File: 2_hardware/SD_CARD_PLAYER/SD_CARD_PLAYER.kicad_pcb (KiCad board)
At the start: 2 copper layers, 142.5 x 128.5 mm, 98 parts, among them J1 Conn_02x05_Odd_Even, J10 SD_CARD_CONN, J11 Analogue Input Jack, J12 Analogue Input Jack, J2 audio output, J3 Digital Input Jack, J4 Digital Input Jack, J5 Digital Input Jack, J7 Digital Input Jack, Q1 MMBT3904, Q2 MMBT3904, Q3 MMBT3904, Q4 MMBT3904, SW1 SW_Push, SW2 SW_Push, SW3 SW_Push, SW4 SW_Push, SW5 SW_SPDT, U1 LM4040DBZ-10, U2 PICO_RP2040, U3 74HC595, U4 MCP6232, U5 LM1117MP-5.0, U6 MCP6002-xMS

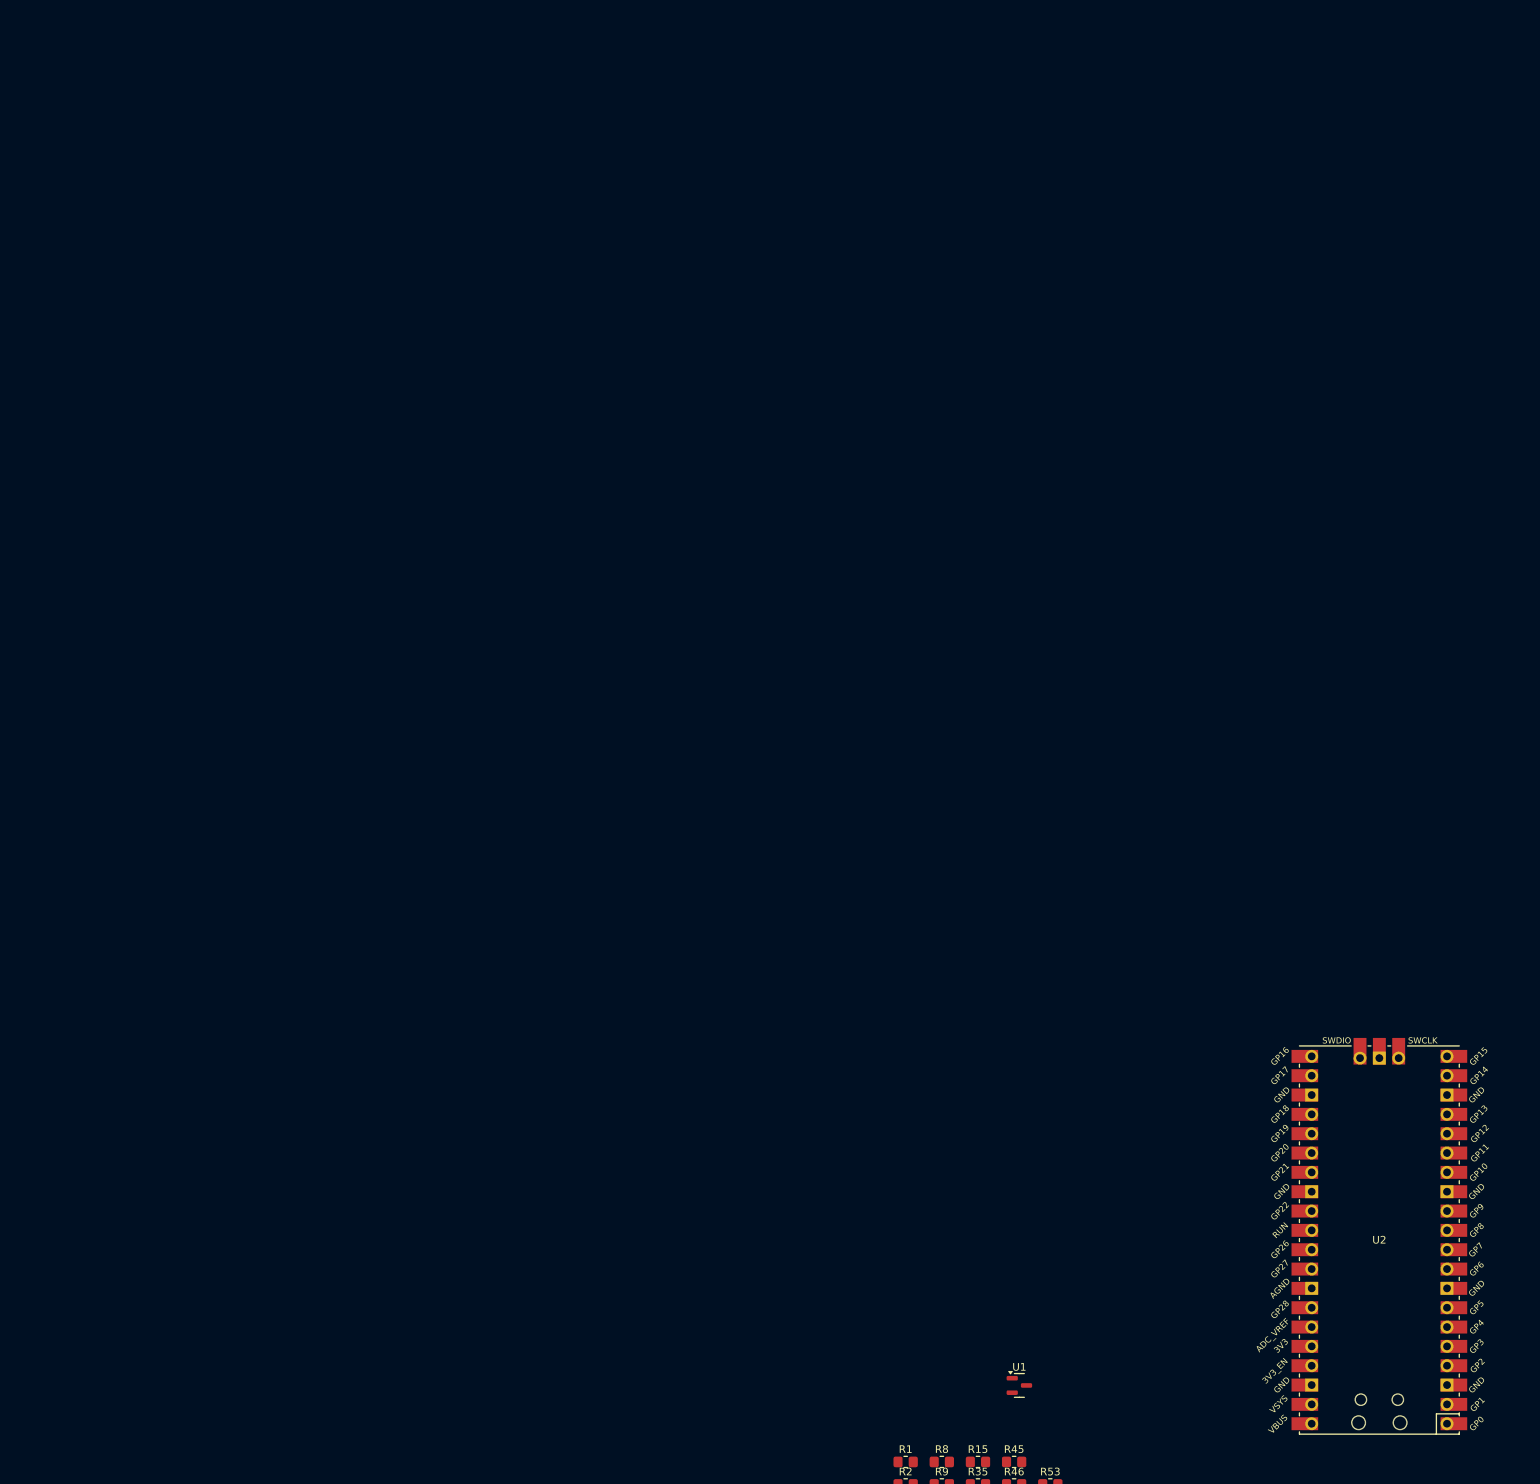
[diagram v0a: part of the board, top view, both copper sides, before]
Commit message: Update test pcb
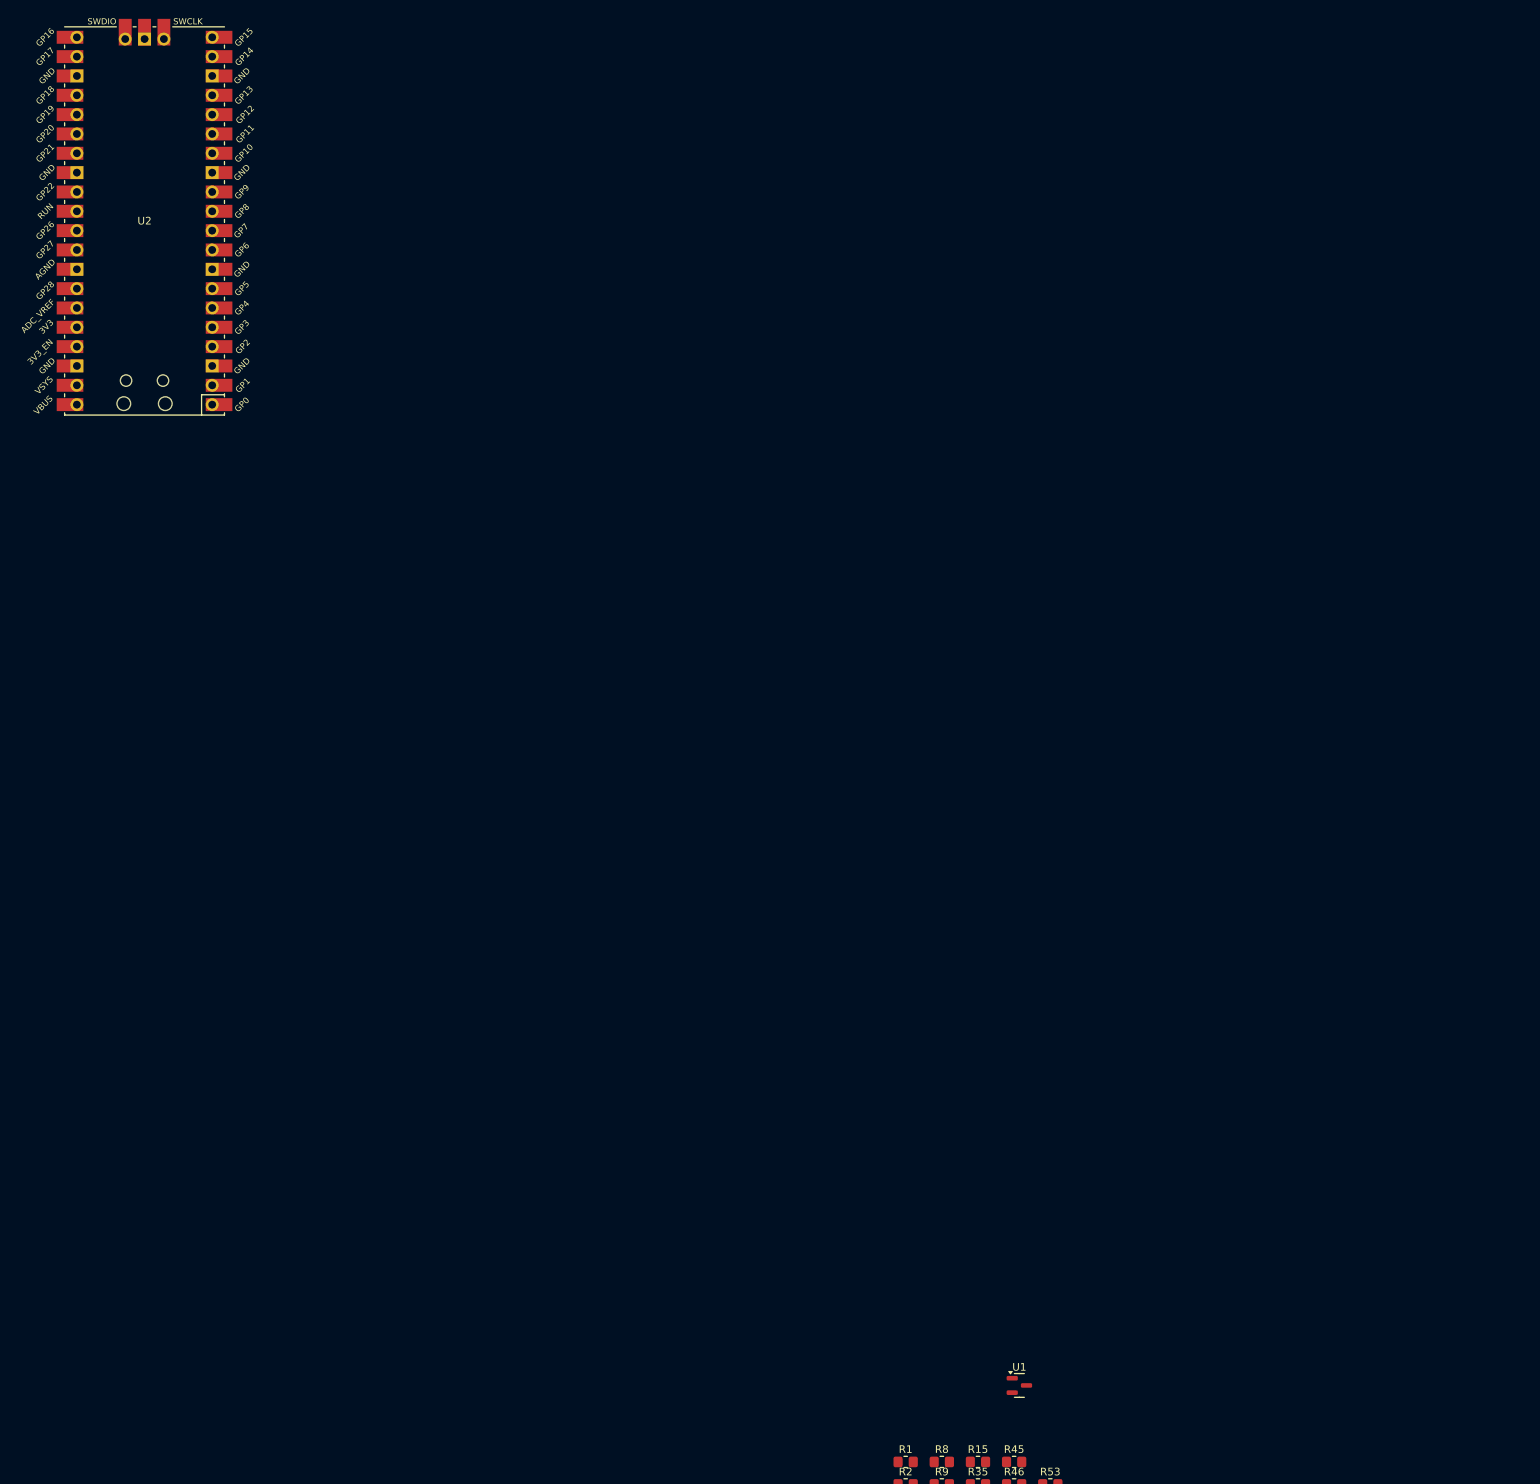
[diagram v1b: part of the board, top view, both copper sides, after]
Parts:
- moved U2 210.3 mm to (-68.0, -44.0)
